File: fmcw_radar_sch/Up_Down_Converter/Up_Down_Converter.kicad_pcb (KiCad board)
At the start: 4 copper layers, 100 x 100 mm, 81 parts, among them J1 Conn_01x04_Pin, J10 Screw_Terminal_01x05, J11 Conn_Coaxial, J12 Conn_Coaxial, J13 Conn_Coaxial, J14 Conn_01x05_Pin, J2 Conn_01x04_Pin, J3 Conn_Coaxial, J4 Conn_01x04_Pin, J5 Conn_01x05_Pin, J6 Conn_Coaxial, J7 Conn_01x01_Pin, J8 USB_C_Receptacle_USB2.0_16P, J9 Screw_Terminal_01x02, SW1 SW_Nidec_CAS-120A1, U1 ADAR2004ACCZ, U3 USBLC6-2SC6, U5 AP63203WU, U6 HT7533-1, U7 ADAR2001ACCZ, U9 ADF4372BCCZ

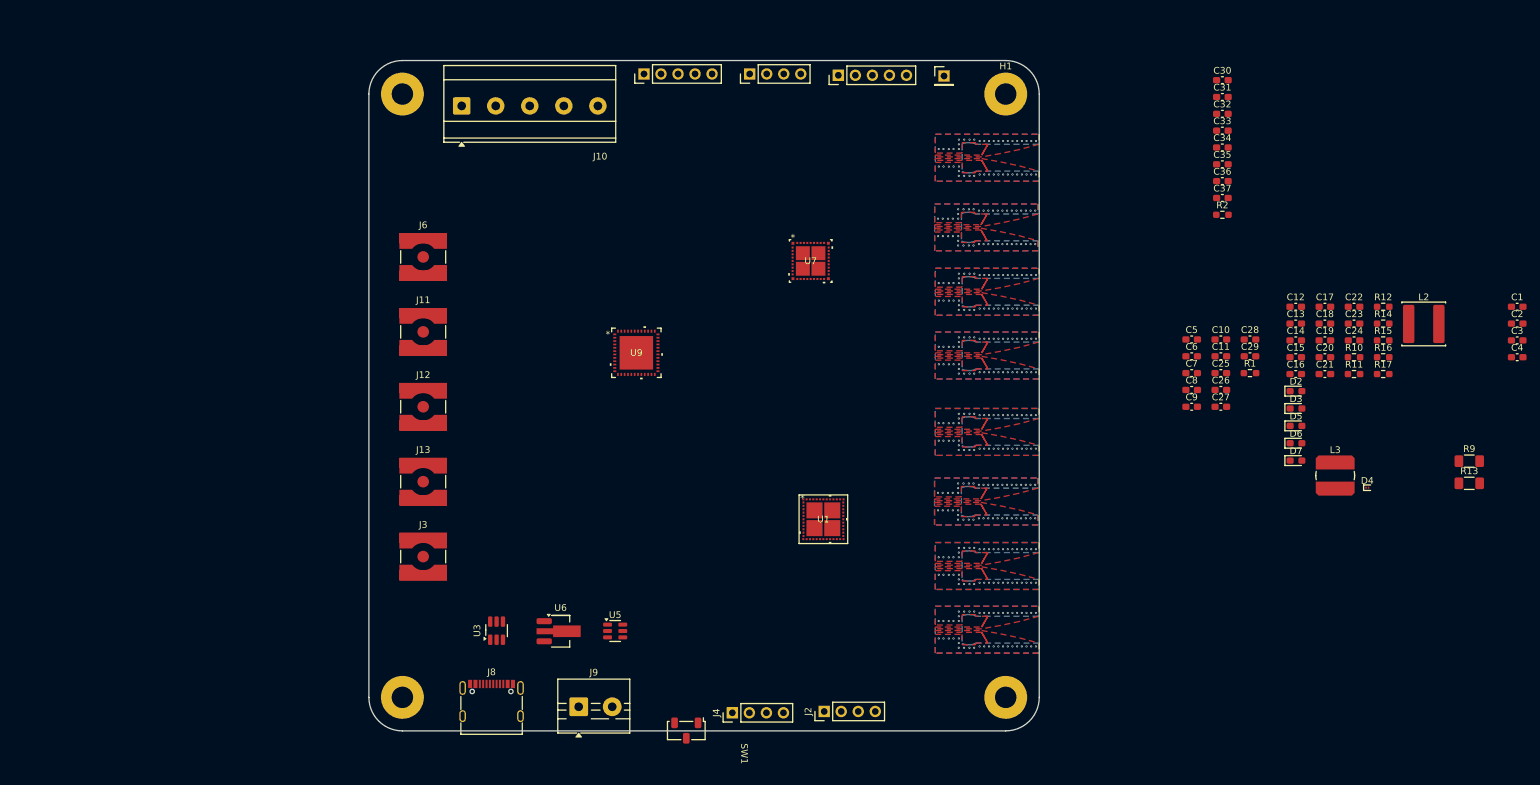
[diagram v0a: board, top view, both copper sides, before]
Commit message: rf changes
rf changes
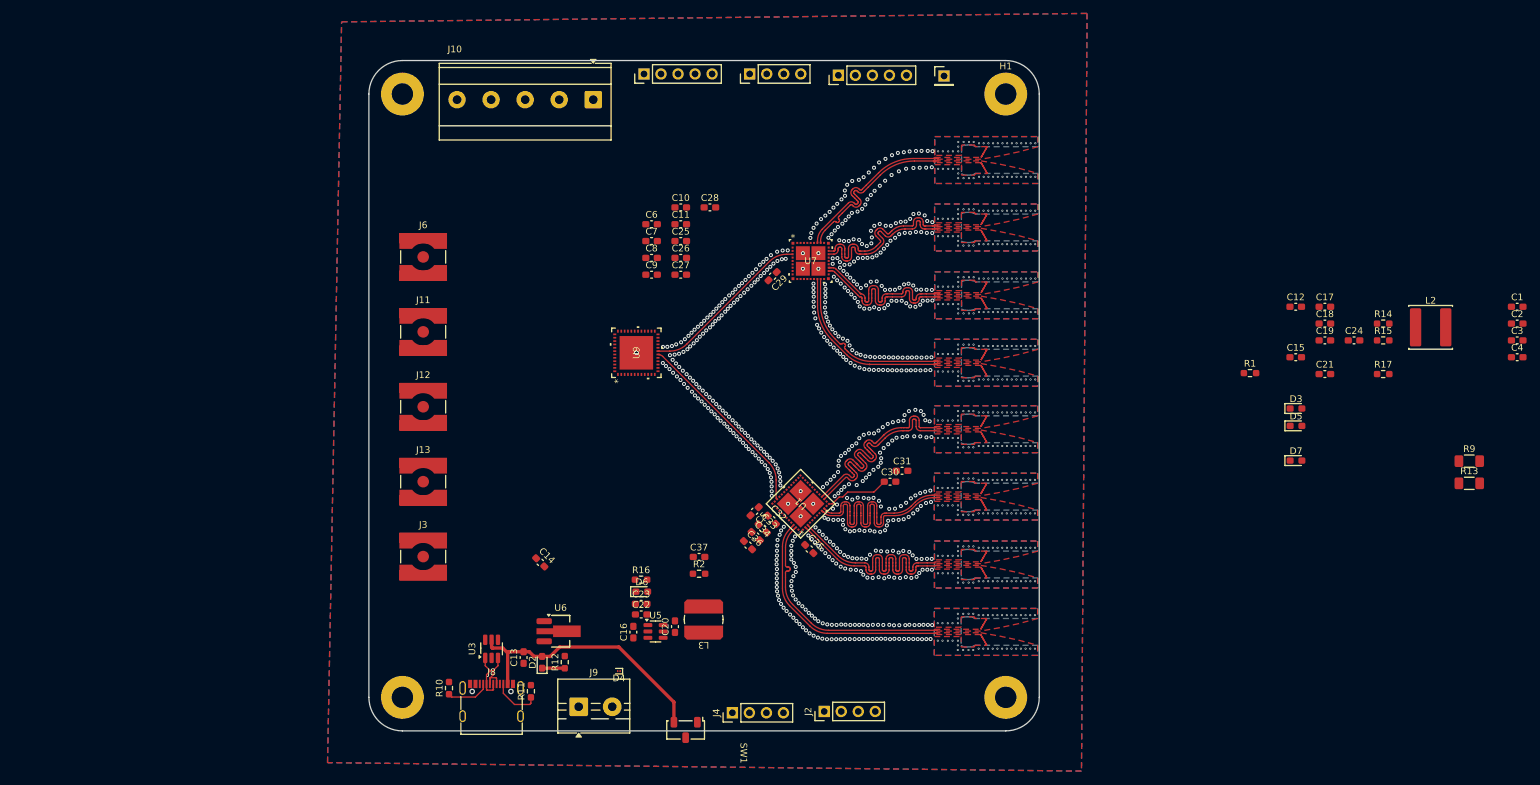
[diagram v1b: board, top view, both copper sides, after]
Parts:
- moved R10 143.8 mm to (112.0, 143.6), turned to 90 degrees
- moved R12 133.1 mm to (129.2, 139.8), turned to 90 degrees
- moved R11 131.6 mm to (124.2, 144.1), turned to 90 degrees
- moved C13 125.5 mm to (123.1, 139.1), turned to 90 degrees
- moved D2 119.5 mm to (125.8, 139.8), turned to 90 degrees
- moved C14 117.5 mm to (125.6, 124.9), turned to -45 degrees
- moved C22 115.8 mm to (140.6, 132.6)
- moved R16 115.6 mm to (140.6, 127.4)
- moved D4 114.9 mm to (137.3, 141.1), turned to 180 degrees
- moved C23 114.3 mm to (140.6, 131.1)
- moved C16 106.0 mm to (139.4, 135.3), turned to 90 degrees
- moved C20 105.0 mm to (145.7, 134.4), turned to 90 degrees
- moved D6 100.1 mm to (140.7, 129.2)
- moved L3 96.6 mm to (149.9, 133.4), turned to 180 degrees
- moved C37 94.7 mm to (149.3, 124.0)
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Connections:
- U1 pad 35: RF8N -> RF8P
- U7 pad 4: RF8P -> RF8N
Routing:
- net VBUS: track 0.00 -> 40.7 mm
- net RFIN1-: track 0.00 -> 36.4 mm
- net RFIN1+: track 0.00 -> 36.3 mm
- net RFIN4-: track 0.00 -> 35.9 mm
- net RFIN3+: track 0.00 -> 35.9 mm
- net RFIN2-: track 0.00 -> 35.8 mm
- net RFIN3-: track 0.00 -> 35.6 mm
- net RFIN4+: track 0.00 -> 35.6 mm
- net RFIN2+: track 0.00 -> 35.4 mm
- net RF8P: track 0.00 -> 29.0 mm
- net RFO1+: track 0.00 -> 26.5 mm
- net RFO1-: track 0.00 -> 26.5 mm
- net RFO3-: track 0.00 -> 26.4 mm
- net RF4O+: track 0.00 -> 26.4 mm
- net RFO2+: track 0.00 -> 26.4 mm
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- added copper zone on B.Cu, net GND
- added copper zone on F.Cu, net GND
- added copper zone on F.Cu, net RF4O+
- added copper zone on F.Cu, net RF4O-
- added copper zone on F.Cu, net RFIN1+
- added copper zone on F.Cu, net RFIN1-
- added copper zone on F.Cu, net RFIN2+
- added copper zone on F.Cu, net RFIN2-
- added copper zone on F.Cu, net RFIN3+
- added copper zone on F.Cu, net RFIN3-
- added copper zone on F.Cu, net RFIN4+
- added copper zone on F.Cu, net RFIN4-
- added copper zone on F.Cu, net RFO1+
- added copper zone on F.Cu, net RFO1-
- added copper zone on F.Cu, net RFO2+
- added copper zone on F.Cu, net RFO2-
- added copper zone on F.Cu, net RFO3+
- added copper zone on F.Cu, net RFO3-
- removed copper zone on F.Cu, net (none)
- removed copper zone on In1.Cu, net (none)

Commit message: changes
changes
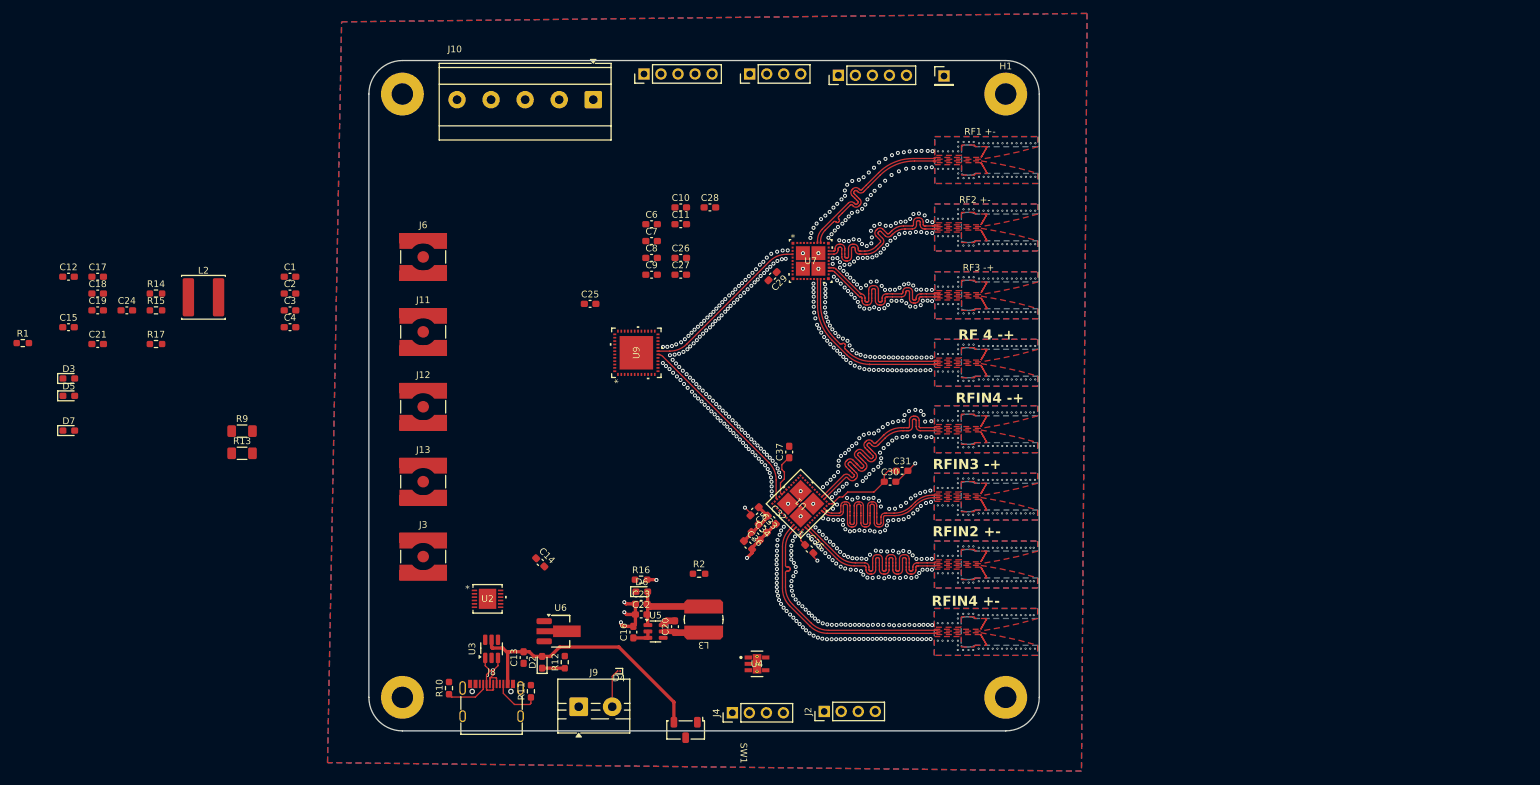
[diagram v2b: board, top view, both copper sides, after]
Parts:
- added U2: LP3875EMP-2.5/NOPB, RF_extra:DNT12_TEX, F.Cu at (117.7, 130.3)
- added U4: TLV75718PDYDR, RF_extra:DYD0005A-MFG, F.Cu at (157.9, 140.0)
- moved C17 183.1 mm to (59.5, 82.2)
- moved C18 183.1 mm to (59.5, 84.8)
- moved C19 183.1 mm to (59.5, 87.3)
- moved C21 183.1 mm to (59.5, 92.3)
- moved C1 183.1 mm to (88.2, 82.2)
- moved C12 183.1 mm to (55.2, 82.2)
- moved C15 183.1 mm to (55.2, 89.8)
- moved C2 183.1 mm to (88.2, 84.8)
- moved C24 183.1 mm to (63.9, 87.3)
- moved C3 183.1 mm to (88.2, 87.3)
- moved C4 183.1 mm to (88.2, 89.8)
- moved D3 183.1 mm to (55.2, 97.4)
- moved D5 183.1 mm to (55.2, 100.0)
- moved D7 183.1 mm to (55.2, 105.2)
- moved L2 183.1 mm to (75.3, 85.3)
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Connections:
- U1 pad 10: RFIN3+ -> GND
- U1 pad 11: RFIN3- -> GND
- U1 pad 15: RFIN4+ -> GND
- U1 pad 16: RFIN4- -> GND
- U1 pad 3: RFIN2- -> GND
- U1 pad 4: RFIN2+ -> GND
- U1 pad 46: RFIN1- -> GND
- U1 pad 47: RFIN1+ -> GND
- U7 pad 18: RF4O+ -> GND
- U7 pad 19: RF4O- -> GND
- U7 pad 23: RFO3+ -> GND
- U7 pad 24: RFO3- -> GND
- U7 pad 28: RFO2- -> GND
- U7 pad 29: RFO2+ -> GND
- U7 pad 33: RFO1- -> GND
- U7 pad 34: RFO1+ -> GND
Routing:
- net GND: track 0.00 -> 520.9 mm, vias 992 -> 999
- net RFIN1-: track 36.4 -> 0.00 mm
- net RFIN1+: track 36.3 -> 0.00 mm
- net RFIN4-: track 35.9 -> 0.00 mm
- net RFIN3+: track 35.9 -> 0.00 mm
- net RFIN2-: track 35.8 -> 0.00 mm
- net RFIN3-: track 35.6 -> 0.00 mm
- net RFIN4+: track 35.6 -> 0.00 mm
- net RFIN2+: track 35.4 -> 0.00 mm
- net RFO1+: track 26.5 -> 0.00 mm
- net RFO1-: track 26.5 -> 0.00 mm
- net RFO3-: track 26.4 -> 0.00 mm
- net RF4O+: track 26.4 -> 0.00 mm
- net RFO2+: track 26.4 -> 0.00 mm
- net RFO2-: track 26.4 -> 0.00 mm
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- removed copper zone on F.Cu, net RFIN1+
- removed copper zone on F.Cu, net RFIN1-
- removed copper zone on F.Cu, net RFIN2+
- removed copper zone on F.Cu, net RFIN2-
- removed copper zone on F.Cu, net RFIN3+
- removed copper zone on F.Cu, net RFIN3-
- removed copper zone on F.Cu, net RFIN4+
- removed copper zone on F.Cu, net RFIN4-
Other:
- board text added: "RF 4 -+"
- board text added: "RF1 +-"
- board text added: "RF2 +-"
- board text added: "RF3 -+"
- board text added: "RFIN2 +-"
- board text added: "RFIN3 -+"
- board text added: "RFIN4 +-"
- board text added: "RFIN4 -+"
